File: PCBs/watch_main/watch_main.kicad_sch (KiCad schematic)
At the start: 1 part, among them U101 Watch_Outline

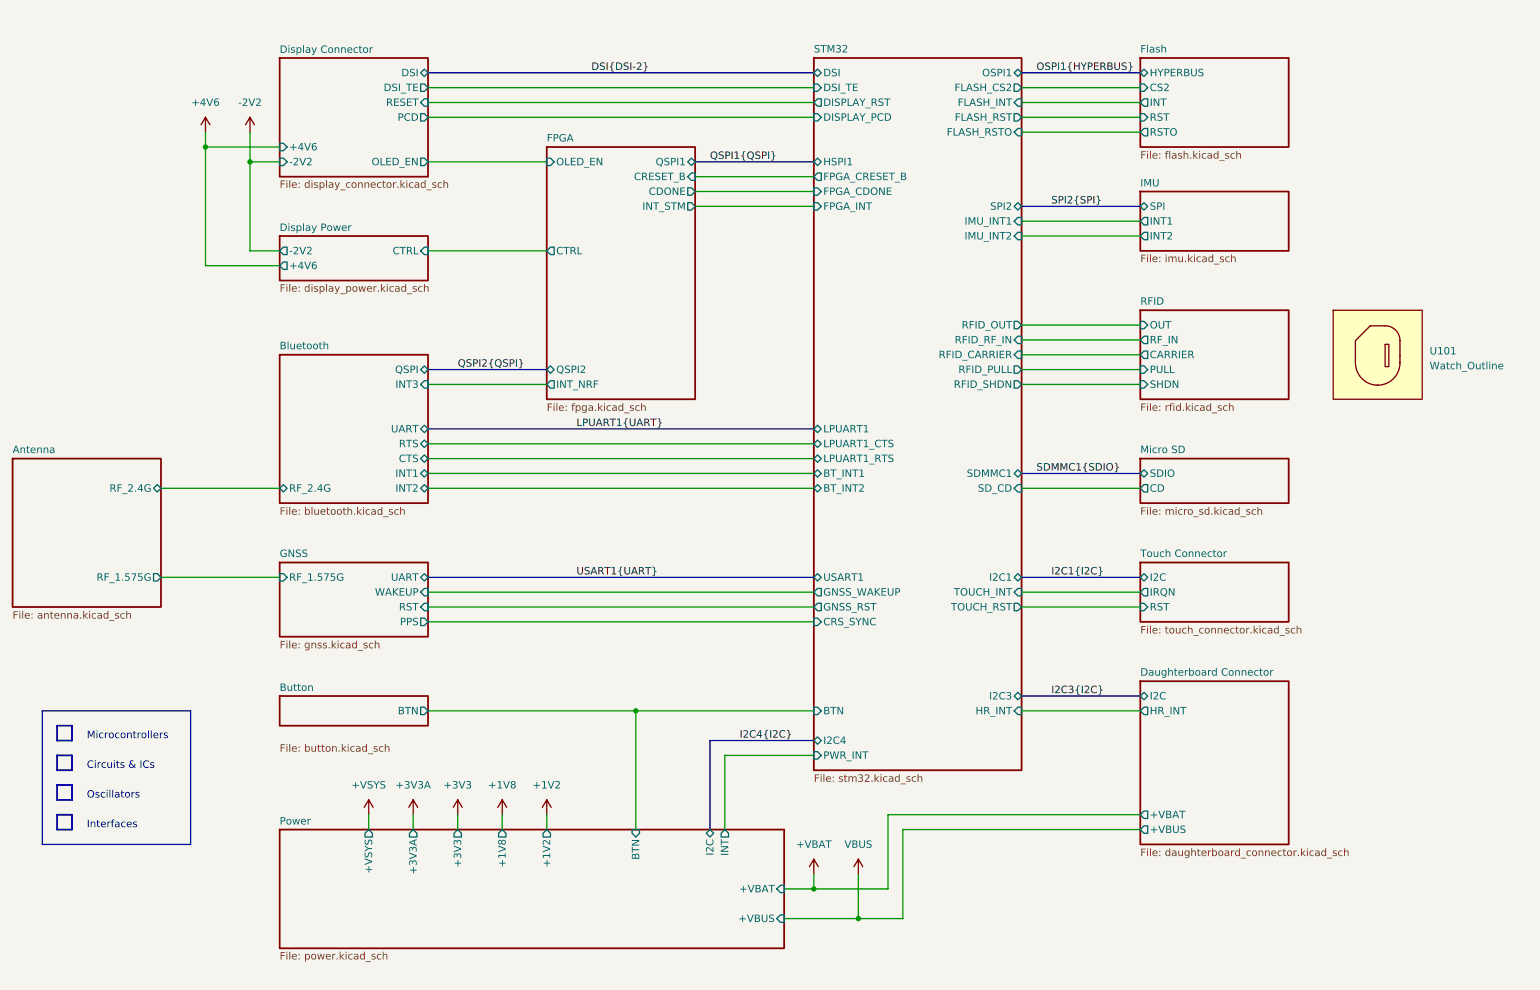
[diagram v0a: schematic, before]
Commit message: Main PCB schematic almost complete
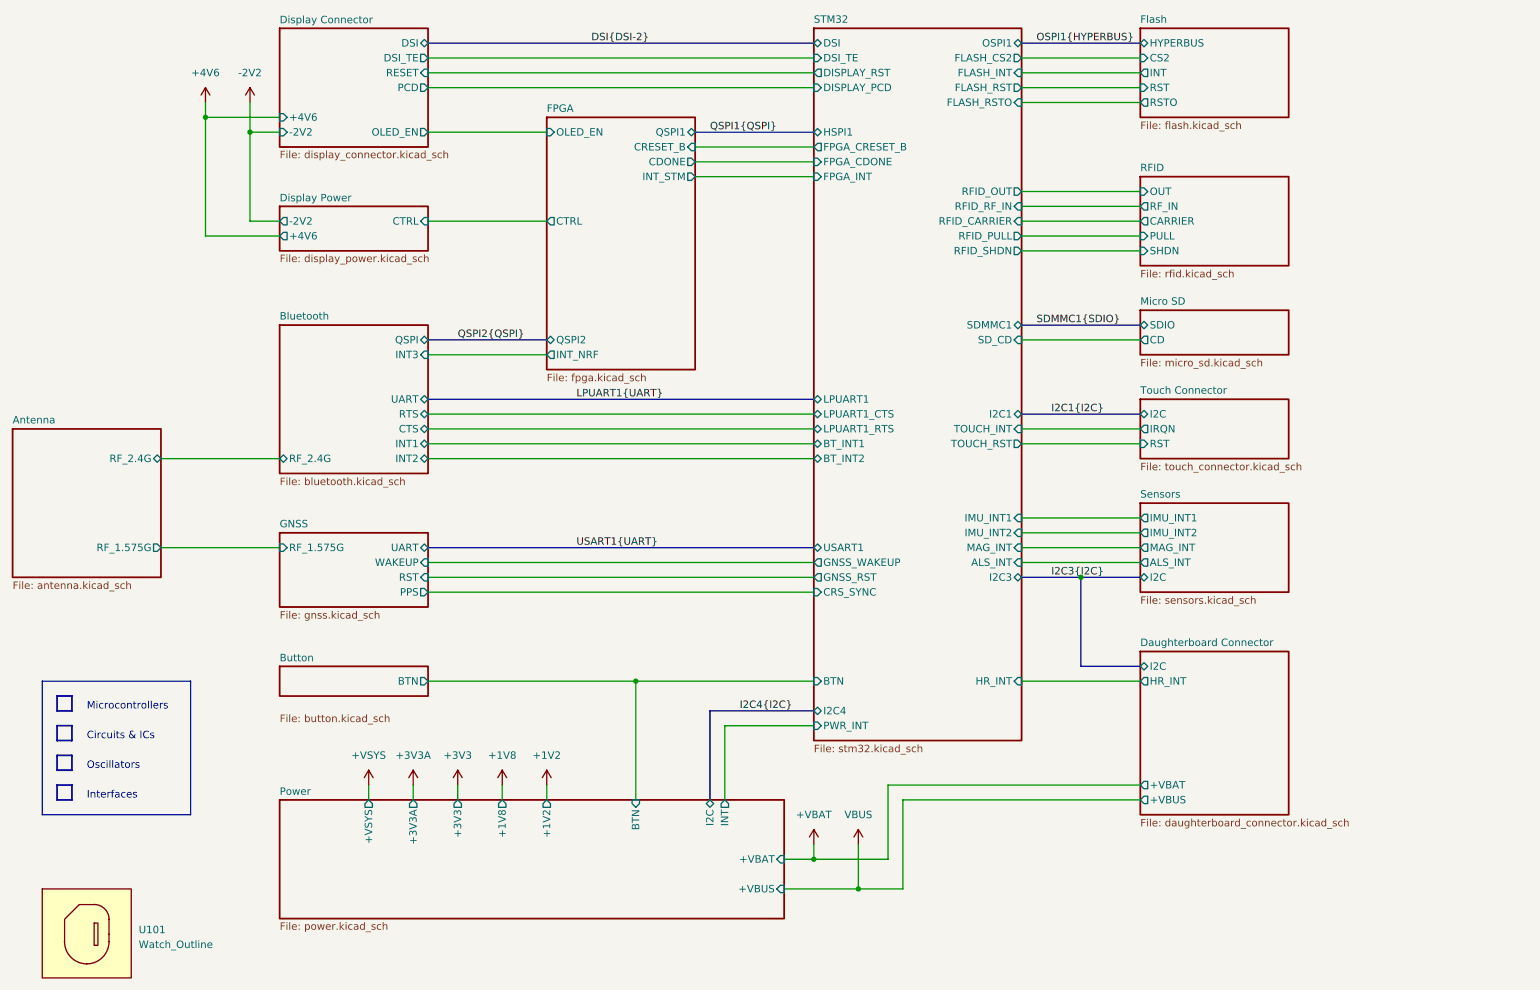
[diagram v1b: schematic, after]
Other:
- removed sheet IMU
- added sheet Sensors (sensors.kicad_sch)
- sheet STM32 ports: added ALS_INT, MAG_INT; removed SPI2
- moved on the sheet: U101
